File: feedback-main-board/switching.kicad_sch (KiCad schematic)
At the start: 39 parts

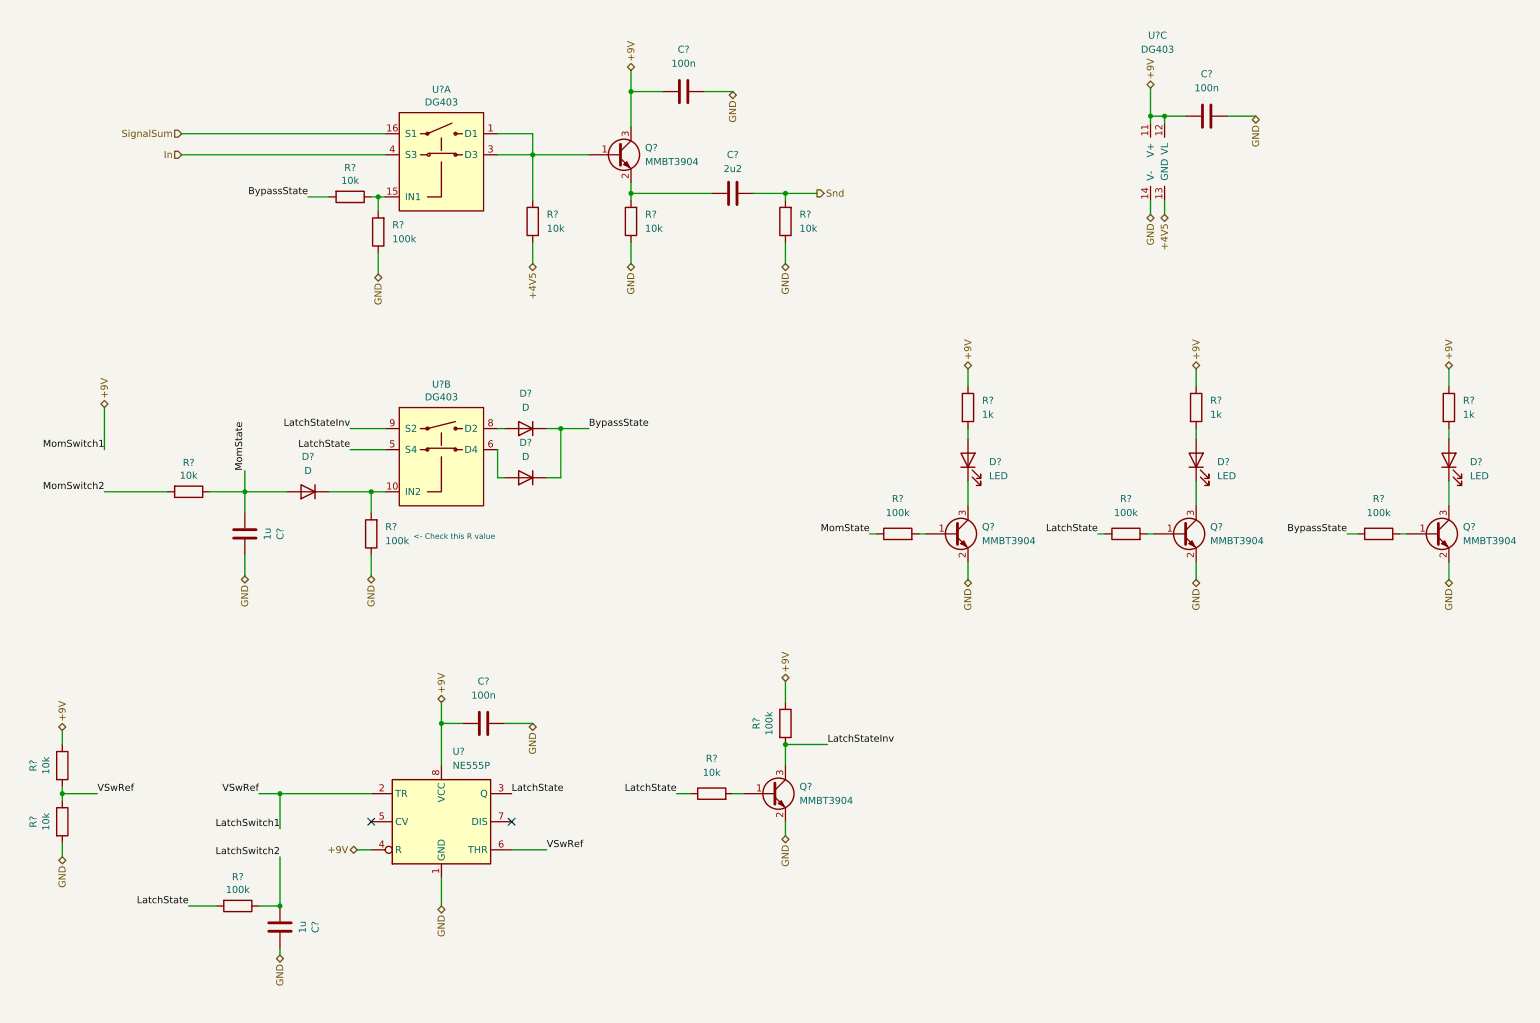
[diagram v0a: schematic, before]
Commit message: Board started
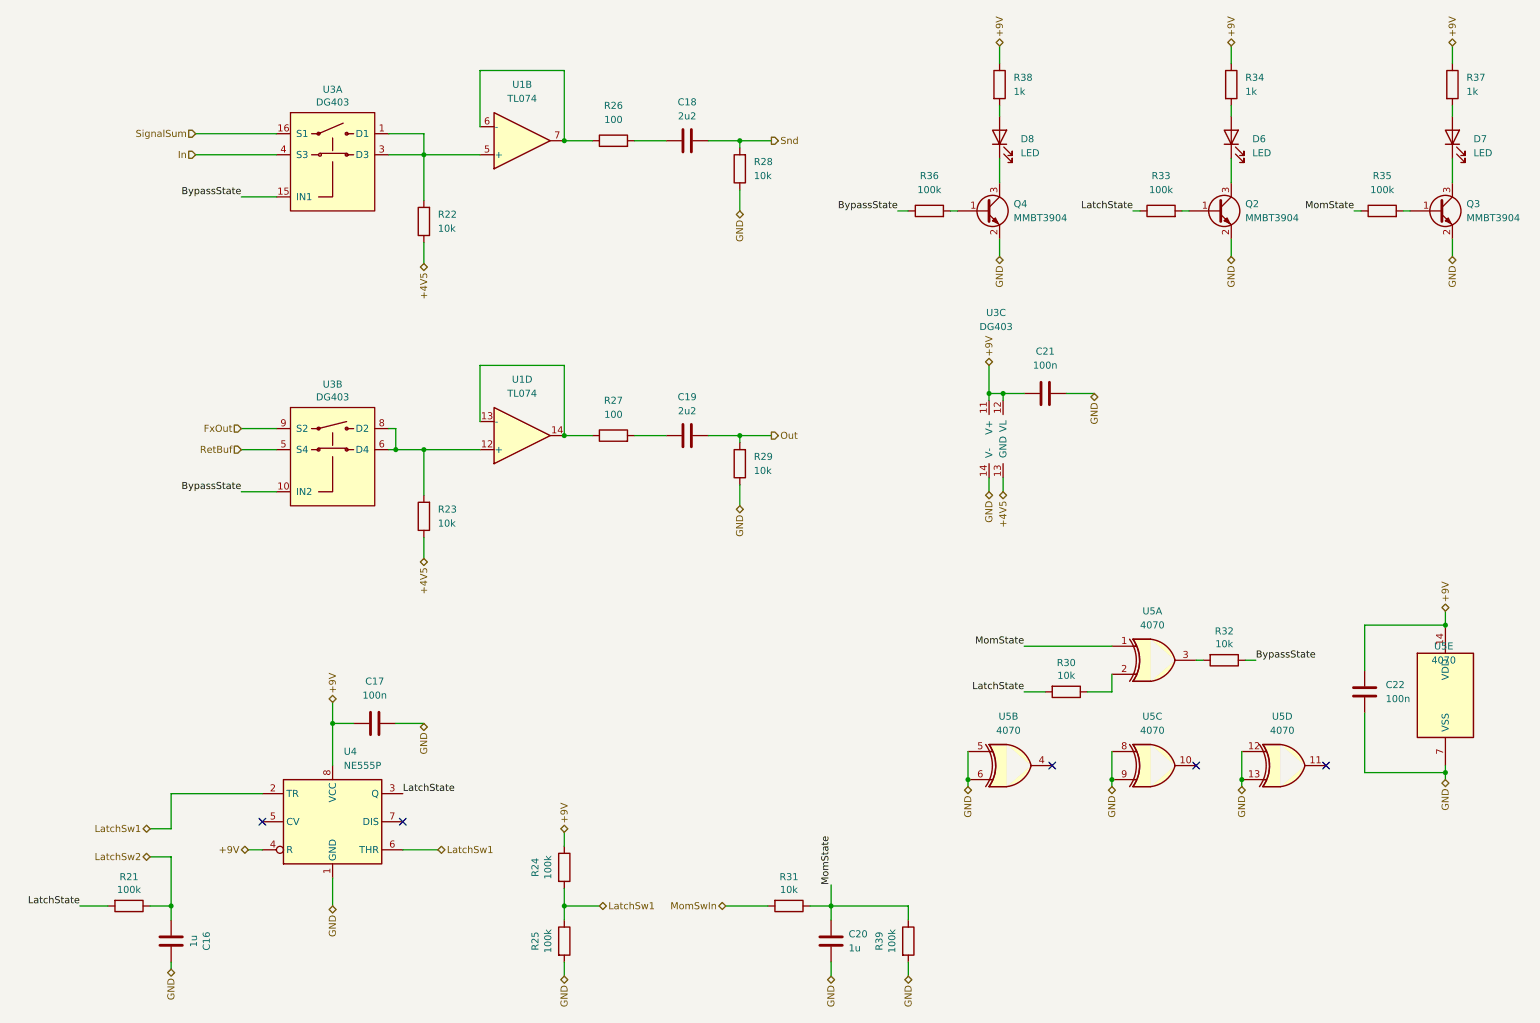
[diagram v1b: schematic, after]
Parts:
- removed C?: 100n, symbol Device:C
- removed C?: 1u, Capacitor_SMD:C_0603_1608Metric_Pad1.08x0.95mm_HandSolder, symbol Device:C
- removed D? (x3): D, symbol Device:D
- removed Q? (x2): MMBT3904, Package_TO_SOT_SMD:SOT-23, symbol Transistor_BJT:MMBT3904
- removed R? (x2): 100k, symbol Device:R
- removed R? (x2): 10k, symbol Device:R
- removed R?: 100k, Resistor_SMD:R_0603_1608Metric_Pad0.98x0.95mm_HandSolder, symbol Device:R
- removed R?: 10k, Resistor_SMD:R_0603_1608Metric_Pad0.98x0.95mm_HandSolder, symbol Device:R
- added C19: 2u2, Capacitor_THT:C_Rect_L7.2mm_W7.2mm_P5.00mm_FKS2_FKP2_MKS2_MKP2, symbol Device:C
- added C20: 1u, Capacitor_SMD:C_0603_1608Metric_Pad1.08x0.95mm_HandSolder, symbol Device:C
- added C22: 100n, Capacitor_SMD:C_0603_1608Metric_Pad1.08x0.95mm_HandSolder, symbol Device:C
- added R23, R29, R30, R32: 10k, Resistor_SMD:R_0603_1608Metric_Pad0.98x0.95mm_HandSolder, symbol Device:R
- added R26, R27: 100, Resistor_SMD:R_0603_1608Metric_Pad0.98x0.95mm_HandSolder, symbol Device:R
- added R39: 100k, Resistor_SMD:R_0603_1608Metric_Pad0.98x0.95mm_HandSolder, symbol Device:R
- added U1: TL074, Package_SO:SOIC-14_3.9x8.7mm_P1.27mm, symbol Amplifier_Operational:TL074
- added U5: 4070, Package_SO:SOIC-14_3.9x8.7mm_P1.27mm, symbol 4xxx:4070
- C17, C21: renamed from C?; footprint (none) -> Capacitor_SMD:C_0603_1608Metric_Pad1.08x0.95mm_HandSolder
- C18: renamed from C?; footprint (none) -> Capacitor_THT:C_Rect_L7.2mm_W7.2mm_P5.00mm_FKS2_FKP2_MKS2_MKP2
- D6, D7, D8: renamed from D?; footprint (none) -> LED_THT:LED_D5.0mm
- R21, R31: renamed from R?; Mouser 603-RT0603DRE07100KL -> (none)
- R22, R28, R33, R35, R36: renamed from R?; footprint (none) -> Resistor_SMD:R_0603_1608Metric_Pad0.98x0.95mm_HandSolder; Mouser 603-RT0603DRE07100KL -> (none)
- R24, R25: renamed from R?; value 10k -> 100k; Mouser 603-RT0603DRE07100KL -> (none)
- R34, R37, R38: renamed from R?; footprint (none) -> Resistor_SMD:R_0603_1608Metric_Pad0.98x0.95mm_HandSolder
- gave numbers to parts that had none: 6
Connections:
- net +4V5: now also R23.1
- net +9V: now also C22.2, U5.14 (VDD)
- net BypassState: now also U3.10 (IN2), U3.15 (IN1), R32.1
- net GND: now also C20.2, C22.1, R29.1, R39.2, U5.12, U5.13, U5.5, U5.6, U5.7 (VSS), U5.8, U5.9
- net LatchState: now also R30.2; no longer U3.5 (S4)
- net MomState: now also C20.1, R39.1, U5.1
- net at U3.6 (D4): now also U3.8 (D2), R23.2, U1.12 (+)
- net at R22.2, U3.1 (D1), U3.3 (D3): now also U1.5 (+)
- net at C18.1: now also R26.2
- net LatchStateInv renamed FxOut
- net LatchSwitch1 renamed LatchSw1
- net LatchSwitch2 renamed LatchSw2
- net MomSwitch2 renamed MomSwIn
- new net: C19.1, R27.2
- new net: R26.1, U1.6 (-), U1.7
- new net: R27.1, U1.13 (-), U1.14
- new net: R32.2, U5.3
- new net: R30.1, U5.2
- new net Out: C19.2, R29.2
- new net RetBuf: U3.5 (S4)
- no-connect marks 2 -> 5
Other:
- note removed: "<- Check this R value"
- moved on the sheet: C16, C17, C18, C21, D6, D7, D8, Q2, Q3, Q4, R21, R22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
